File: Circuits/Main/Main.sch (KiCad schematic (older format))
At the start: 56 parts, among them P1 led_stop, P10 toEncoder_MotorL, P11 toEncoder_motorR, P2 led_droite_face, P3 led_droite_cote, P4 led_gauche_face, P5 led_gauche_cote, U1 beagleBone, U2 NandBuffer

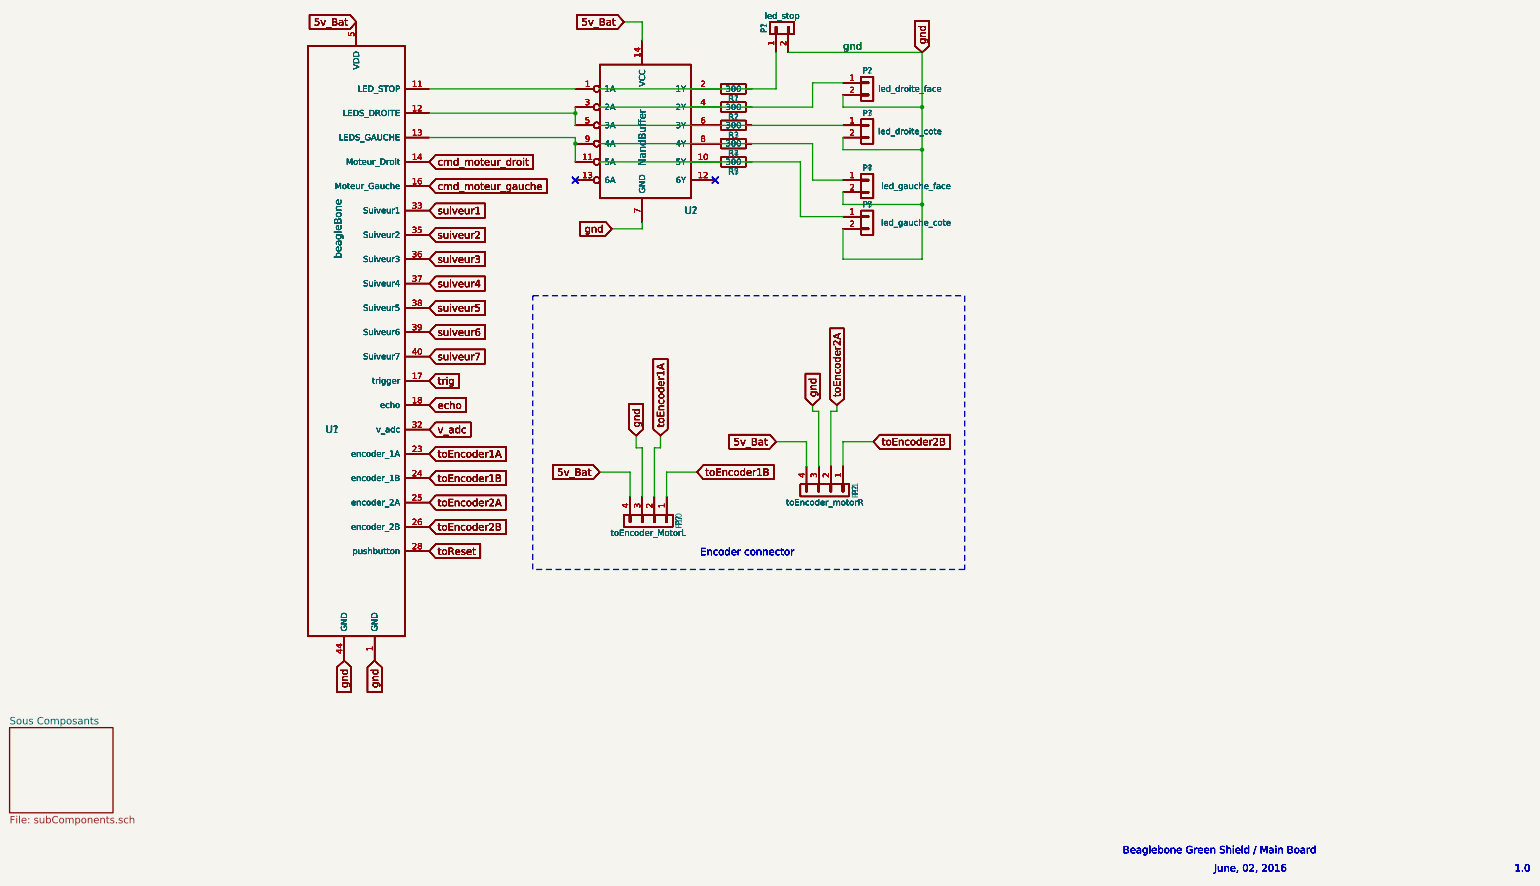
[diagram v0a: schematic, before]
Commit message: Ameliorations cartes + rapport
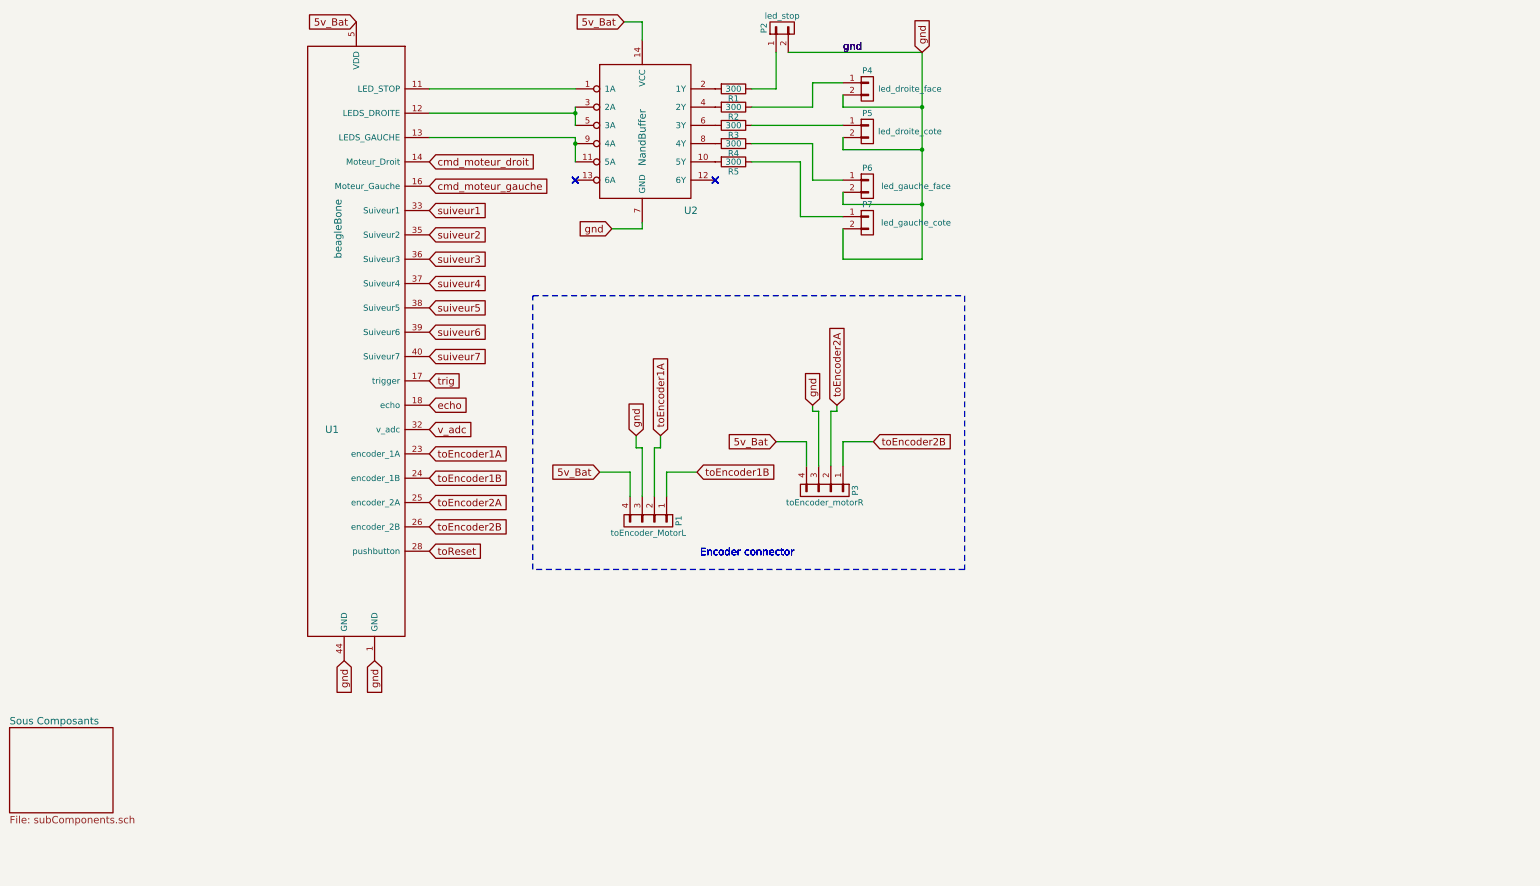
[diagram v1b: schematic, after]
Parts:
- removed P10, P? (x2): toEncoder_MotorL, Pin_Headers:Pin_Header_Straight_1x04, symbol CONN_01X04
- removed P? (x3): led_stop, Pin_Headers:Pin_Header_Straight_1x02, symbol CONN_01X02
- removed P? (x3): led_gauche_cote, Pin_Headers:Pin_Header_Straight_1x02, symbol CONN_01X02
- removed P? (x3): led_gauche_face, Pin_Headers:Pin_Header_Straight_1x02, symbol CONN_01X02
- removed P? (x3): led_droite_face, Pin_Headers:Pin_Header_Straight_1x02, symbol CONN_01X02
- removed P? (x3): led_droite_cote, Pin_Headers:Pin_Header_Straight_1x02, symbol CONN_01X02
- removed P? (x3): toEncoder_motorR, Pin_Headers:Pin_Header_Straight_1x04, symbol CONN_01X04
- removed R? (x15): 300, Resistors_ThroughHole:Resistor_Horizontal_RM10mm, symbol R
- removed U? (x3): NandBuffer, MES_EMPREINTES:NandBuffer, symbol NandBuffer
- removed U? (x3): beagleBone, MES_EMPREINTES:beagleBoneGRNFootPrint, symbol beagleBone
- gave numbers to parts that had none: 1
- renumbered P1 to P2, P11 to P3, P2 to P4, P3 to P5, P4 to P6, P5 to P7
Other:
- note removed: "1.0"
- note removed: "Beaglebone Green Shield / Main Board"
- note removed: "June, 02, 2016"
